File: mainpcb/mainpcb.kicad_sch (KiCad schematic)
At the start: 7 parts, among them J1 Raspberry_Pi_2_3, J3 8P8C_Shielded, J8 8P8C_Shielded, J9 Screw_Terminal_01x09, U4 TXB0108PW, U5 TCA9517ADGK

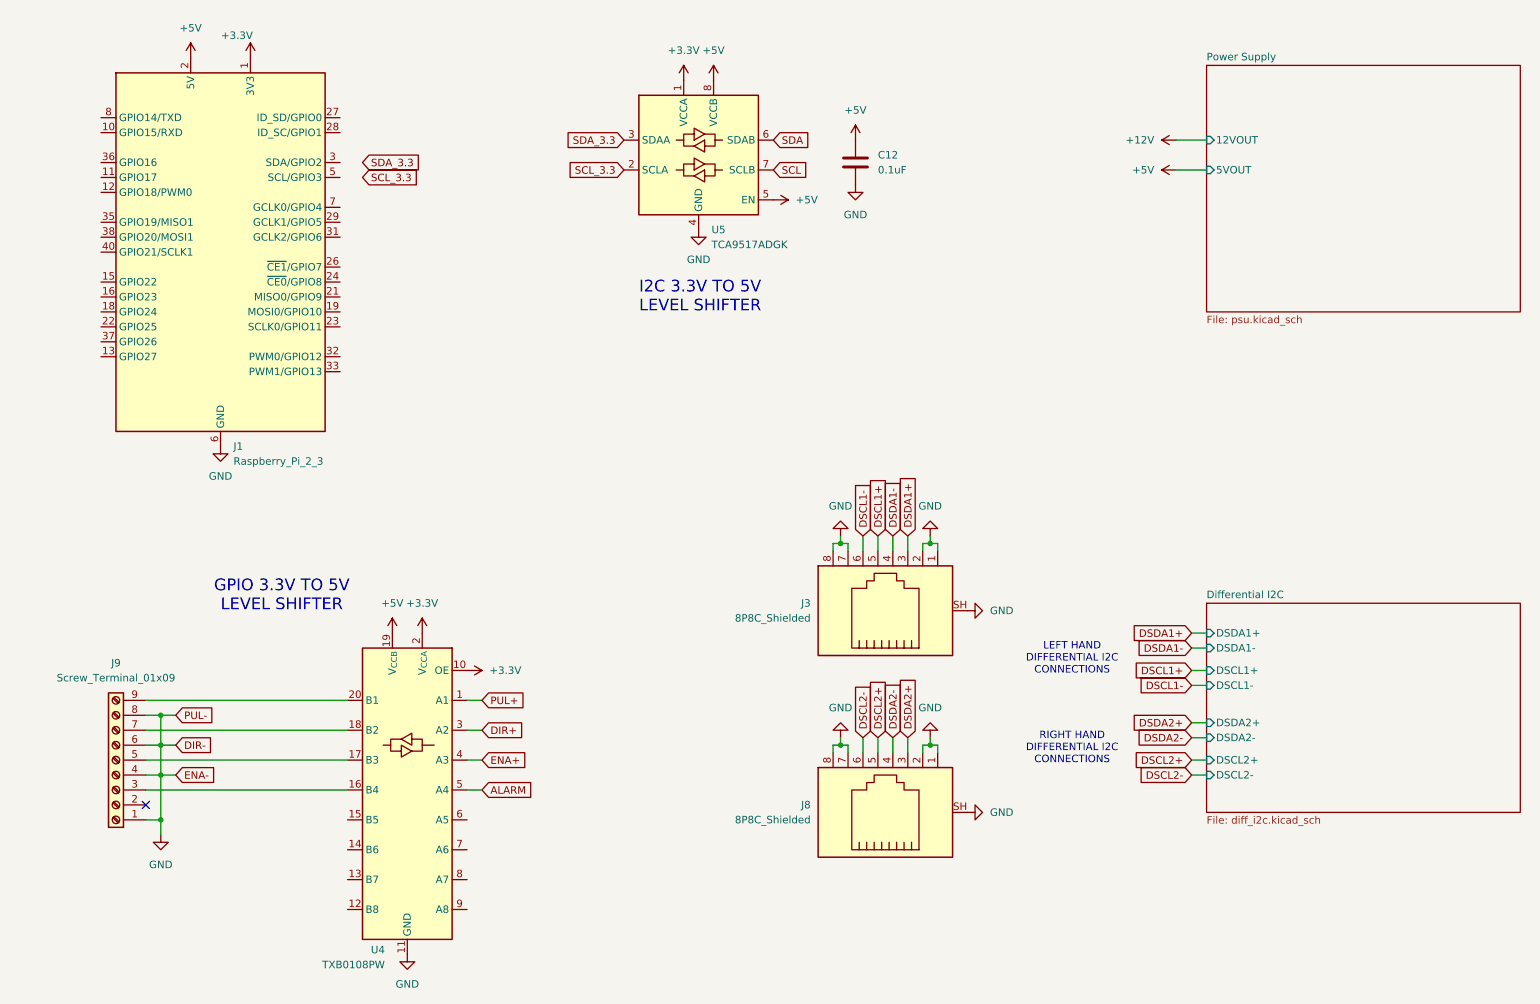
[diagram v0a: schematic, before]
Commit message: Major update
Hand PCB mostly complete
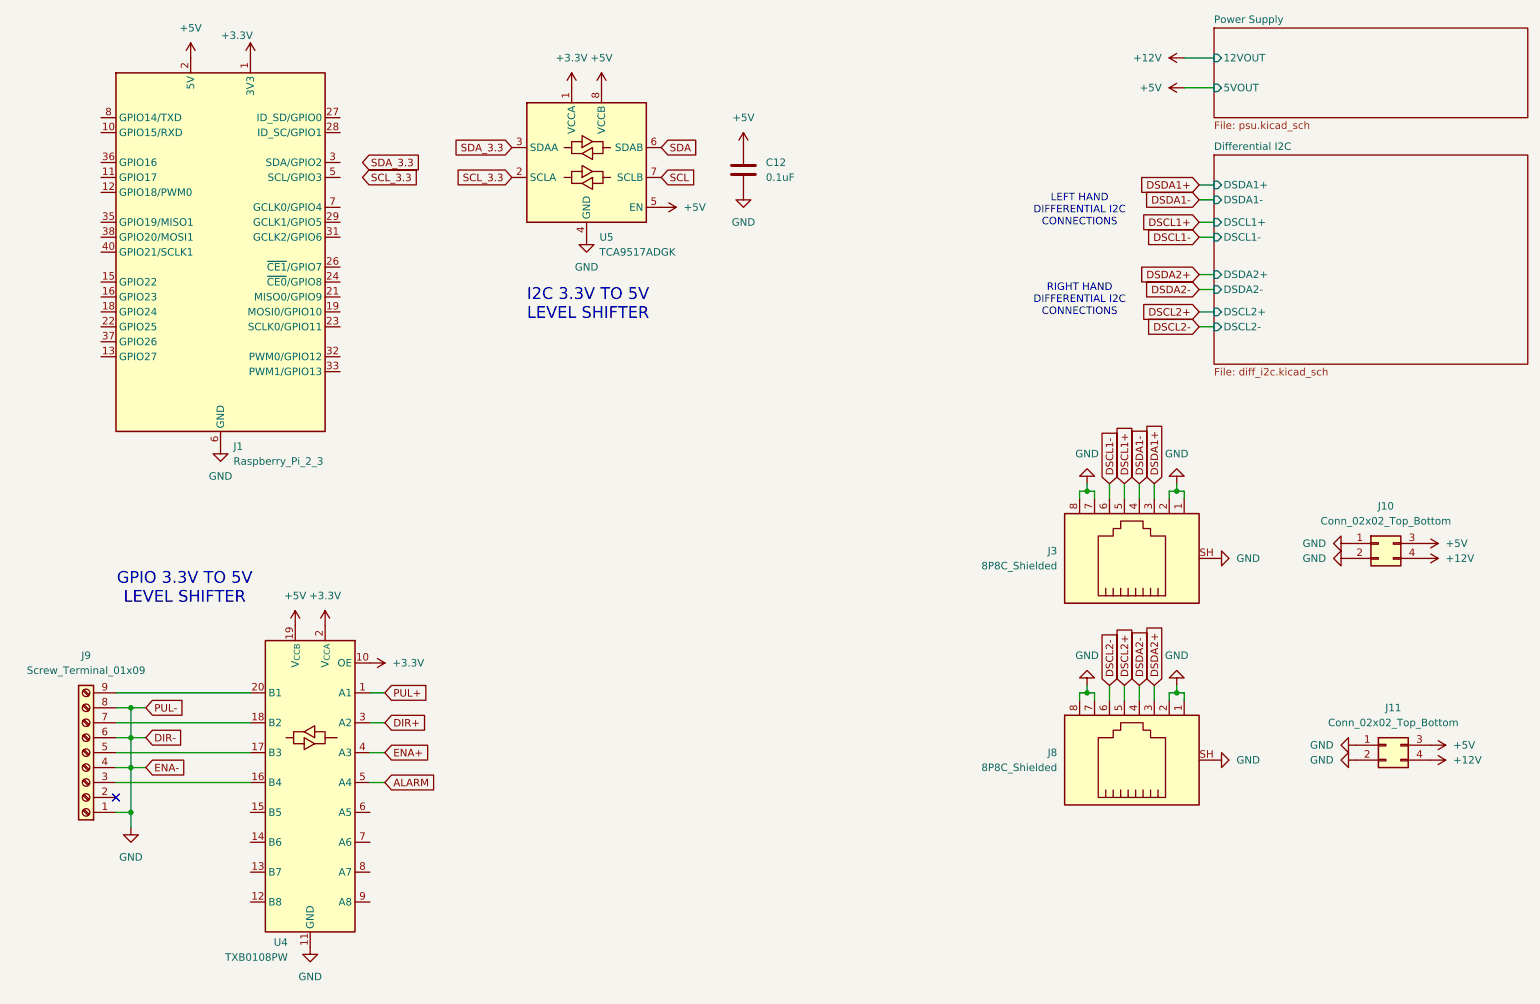
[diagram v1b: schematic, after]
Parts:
- added J10, J11: Conn_02x02_Top_Bottom, Connector_Molex:Molex_Mini-Fit_Jr_5569-04A2_2x02_P4.20mm_Horizontal, symbol Connector_Generic:Conn_02x02_Top_Bottom
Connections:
- net +12V: now also J10.4 (Pin_4), J11.4 (Pin_4)
- net +5V: now also J10.3 (Pin_3), J11.3 (Pin_3)
- net GND: now also J10.1 (Pin_1), J10.2 (Pin_2), J11.1 (Pin_1), J11.2 (Pin_2)
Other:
- moved on the sheet: C12, J3, J8, J9, U4, U5
